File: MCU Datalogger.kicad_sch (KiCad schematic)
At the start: 25 parts, among them U1 24LC1025, U2 24LC1025, U3 DS1337S_T_R, U4 ATMEGA328P-AN, Y1 32.768 KHz, Y2 16 MHz

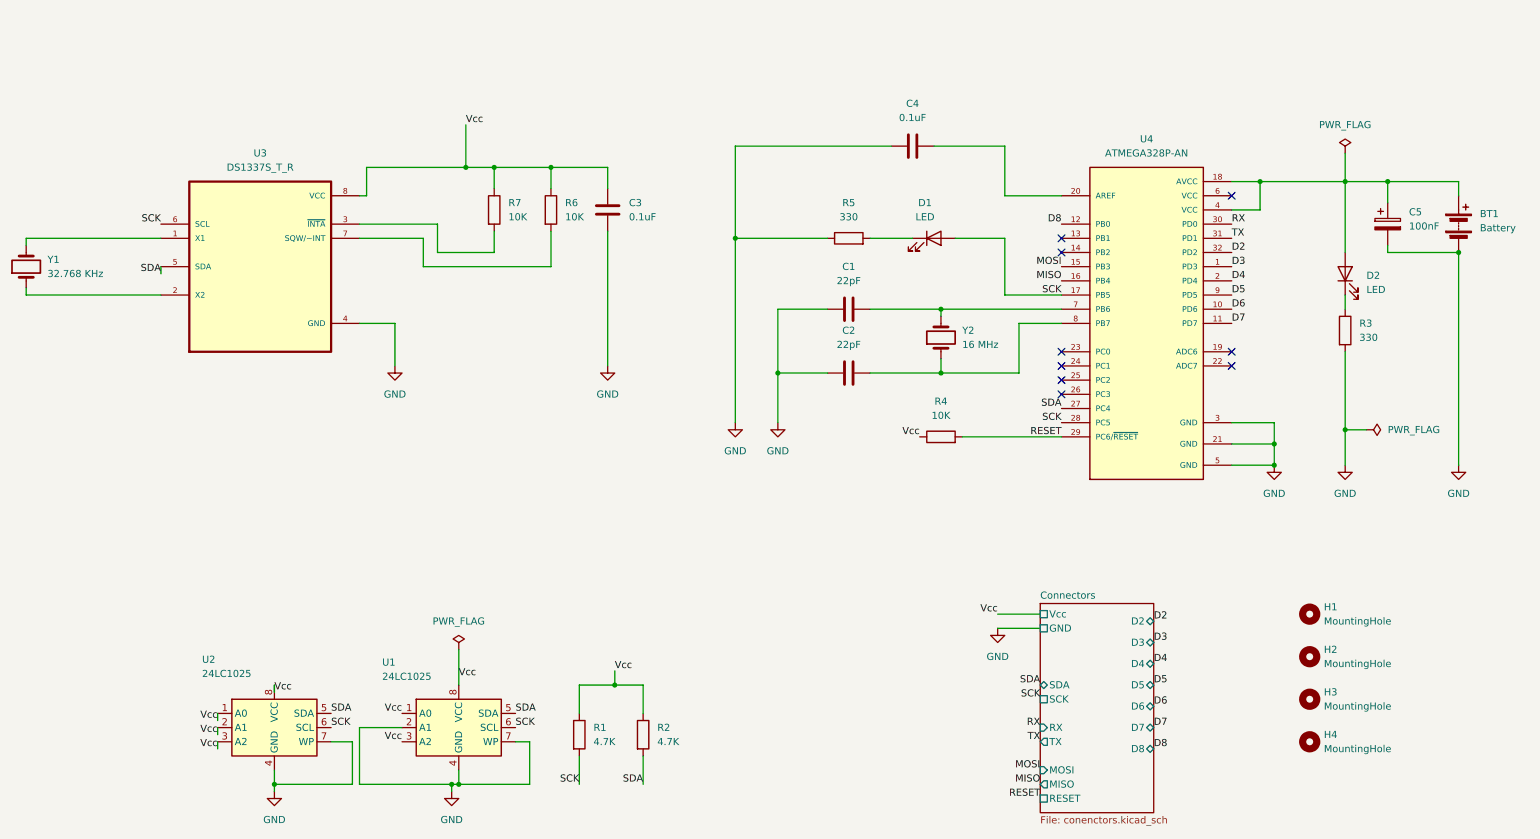
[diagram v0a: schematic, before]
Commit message: fix bugs
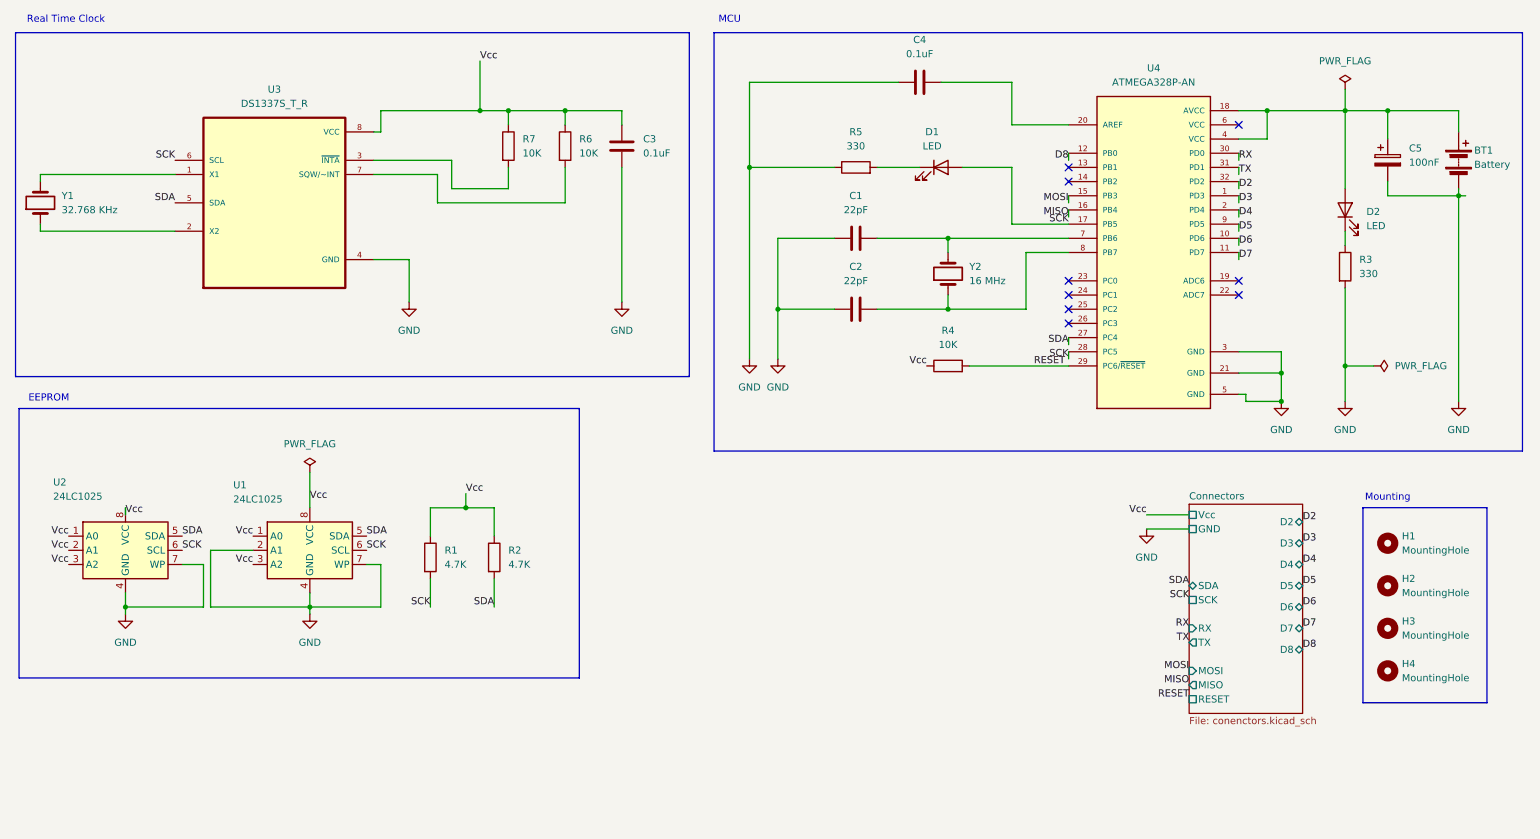
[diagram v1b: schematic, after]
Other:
- note added: "EEPROM"
- note added: "MCU"
- note added: "Mounting"
- note added: "Real Time Clock"
- moved on the sheet: BT1, C1, C2, C3, C4, C5, D1, D2, H1, H2, H3, H4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
